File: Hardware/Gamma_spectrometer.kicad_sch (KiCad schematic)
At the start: 62 parts, among them J1 Conn_01x04, J11 Test Pad, J2 Conn_01x04, J3 Conn_01x01, J4 Conn_01x04, J5 Test Pad, J6 Test Pad, J7 Test Pad, J8 Test Pad, J9 Test Pad, Q1 2N7002, U1 74VHC9164FT, U11 ATtiny1616-M, U2 LM317L_SO8, U3 OPA356xxDBV, U4 OPA355NA, U5 OPA355NA, U6 LMV7219M7, U7 OPA356xxDBV, U8 FODM217A

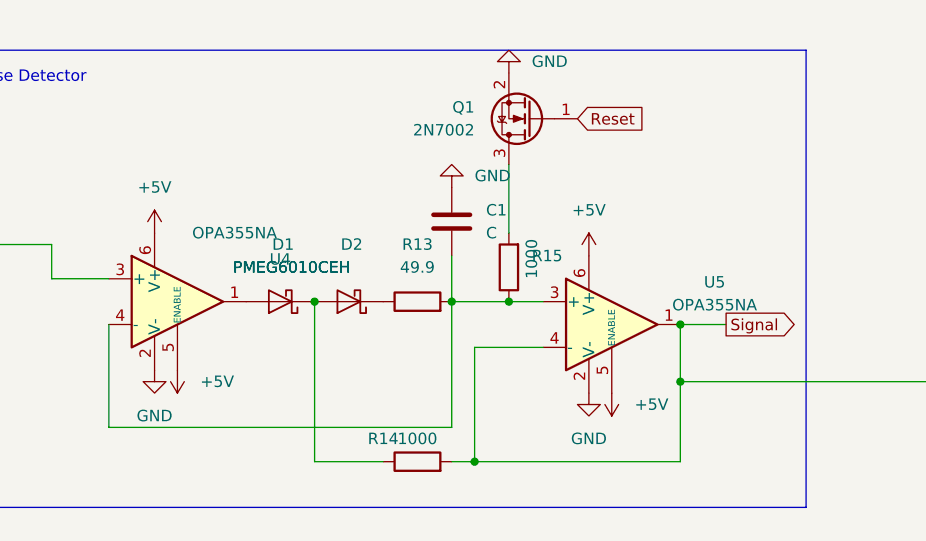
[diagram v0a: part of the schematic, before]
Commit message: BOM scv update
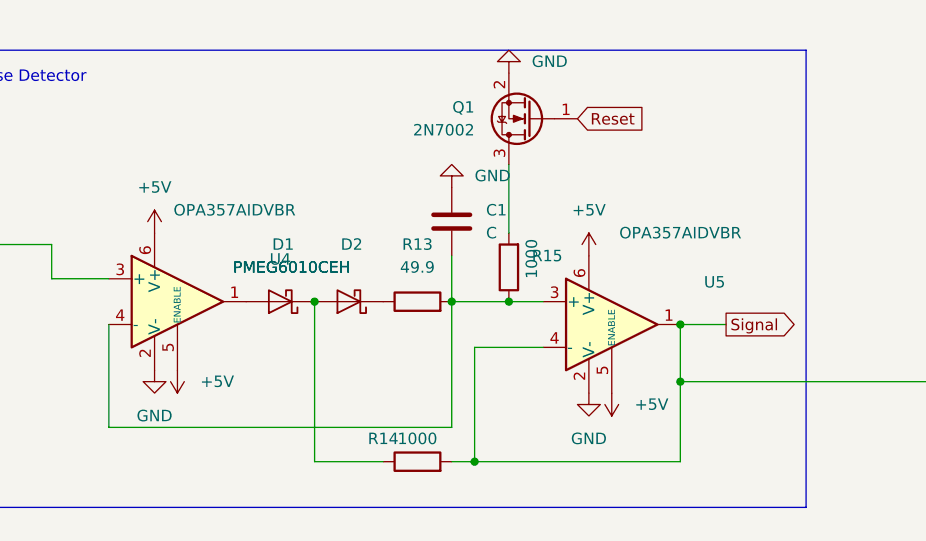
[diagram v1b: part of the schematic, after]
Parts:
- U4, U5: value OPA355NA -> OPA357AIDVBR
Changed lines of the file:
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@@
     (in_bom yes) (on_board yes)
     (property "Reference" "U4" (id 0) (at 175.26 35.941 0))
-    (property "Value" "OPA355NA" (id 1) (at 170.18 33.02 0))
+    (property "Value" "OPA357AIDVBR" (id 1) (at 170.18 30.48 0))
     (property "Footprint" "Package_TO_SOT_SMD:SOT-23-6" (id 2) (at 167.64 46.99 0)
       (effects (font (size 1.27 1.27)) (justify left) hide)
@@
   )
   (symbol (lib_id "Amplifier_Operational:OPA355NA") (at 212.09 43.18 0) (unit 1)
-    (in_bom yes) (on_board yes) (fields_autoplaced)
+    (in_bom yes) (on_board yes)
     (property "Reference" "U5" (id 0) (at 223.52 38.481 0))
-    (property "Value" "OPA355NA" (id 1) (at 223.52 41.021 0))
+    (property "Value" "OPA357AIDVBR" (id 1) (at 219.71 33.02 0))
     (property "Footprint" "Package_TO_SOT_SMD:SOT-23-6" (id 2) (at 215.9 49.53 0)
       (effects (font (size 1.27 1.27)) (justify left) hide)
@@
     )
     (path "/16e3266a-fa79-4a13-8a63-262ef7365400"
-      (reference "U4") (unit 1) (value "OPA355NA") (footprint "Package_TO_SOT_SMD:SOT-23-6")
+      (reference "U4") (unit 1) (value "OPA357AIDVBR") (footprint "Package_TO_SOT_SMD:SOT-23-6")
     )
     (path "/bd06f070-6e8d-4cf0-b42c-cfecd325cf98"
-      (reference "U5") (unit 1) (value "OPA355NA") (footprint "Package_TO_SOT_SMD:SOT-23-6")
+      (reference "U5") (unit 1) (value "OPA357AIDVBR") (footprint "Package_TO_SOT_SMD:SOT-23-6")
     )
     (path "/9142b0ff-741b-4445-9ab6-e977730a6c9f"
